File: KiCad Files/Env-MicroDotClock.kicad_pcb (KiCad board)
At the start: 2 copper layers, 90 x 65.2 mm, 48 parts, among them IC1 IS31FL3730-QFLS2-TR, IC2 IS31FL3730-QFLS2-TR, IC3 IS31FL3730-QFLS2-TR, IC4 IS31FL3730-QFLS2-TR, M1 Dip-14 Socket, M2 Dip-14 Socket, M3 Dip-14 Socket, M4 Dip-14 Socket, M5 Dip-14 Socket, M6 Dip-14 Socket, M7 Dip-14 Socket, M8 Dip-14 Socket, Q1 2SC1815, SW1 SKRK, SW2 SKRK, SW3 SKRK, SW4 SKRK, U1 Raspberry Pi Pico, U3 DS3231M

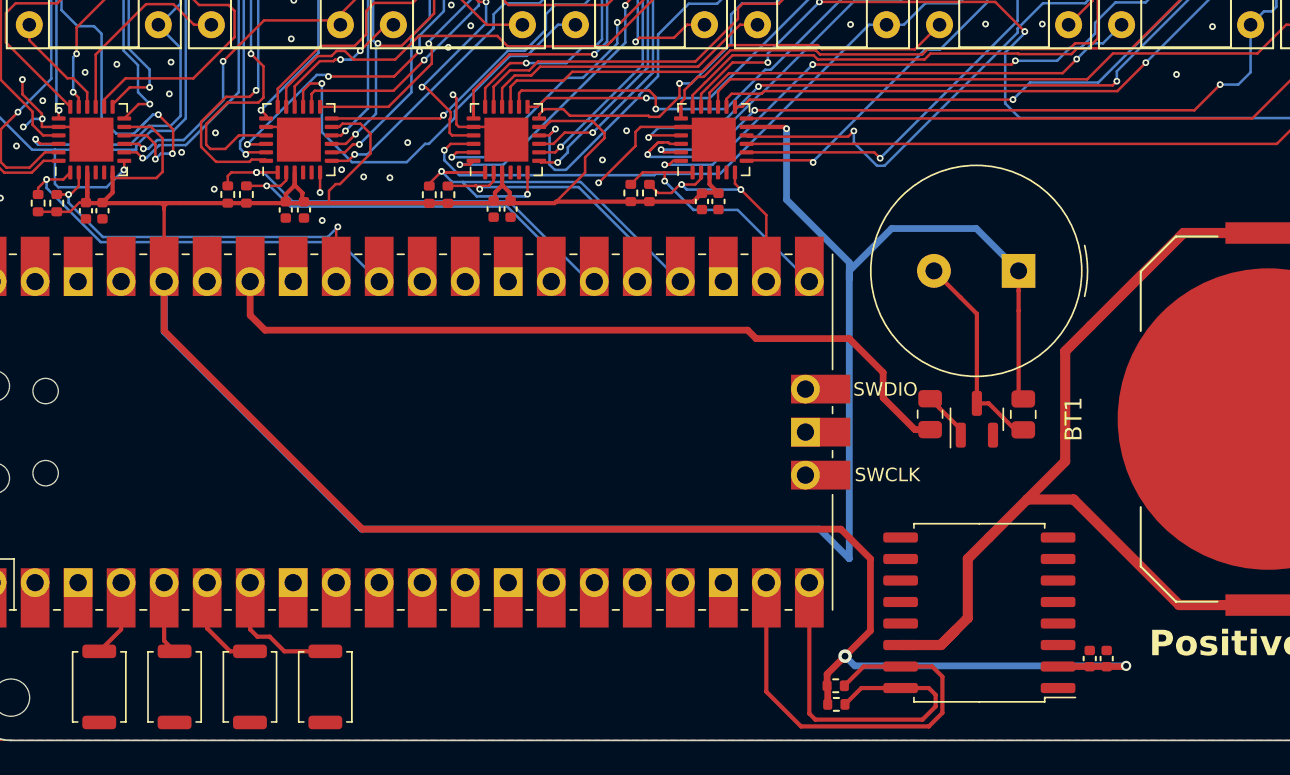
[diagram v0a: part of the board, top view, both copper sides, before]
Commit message: small tweaks + generated production files
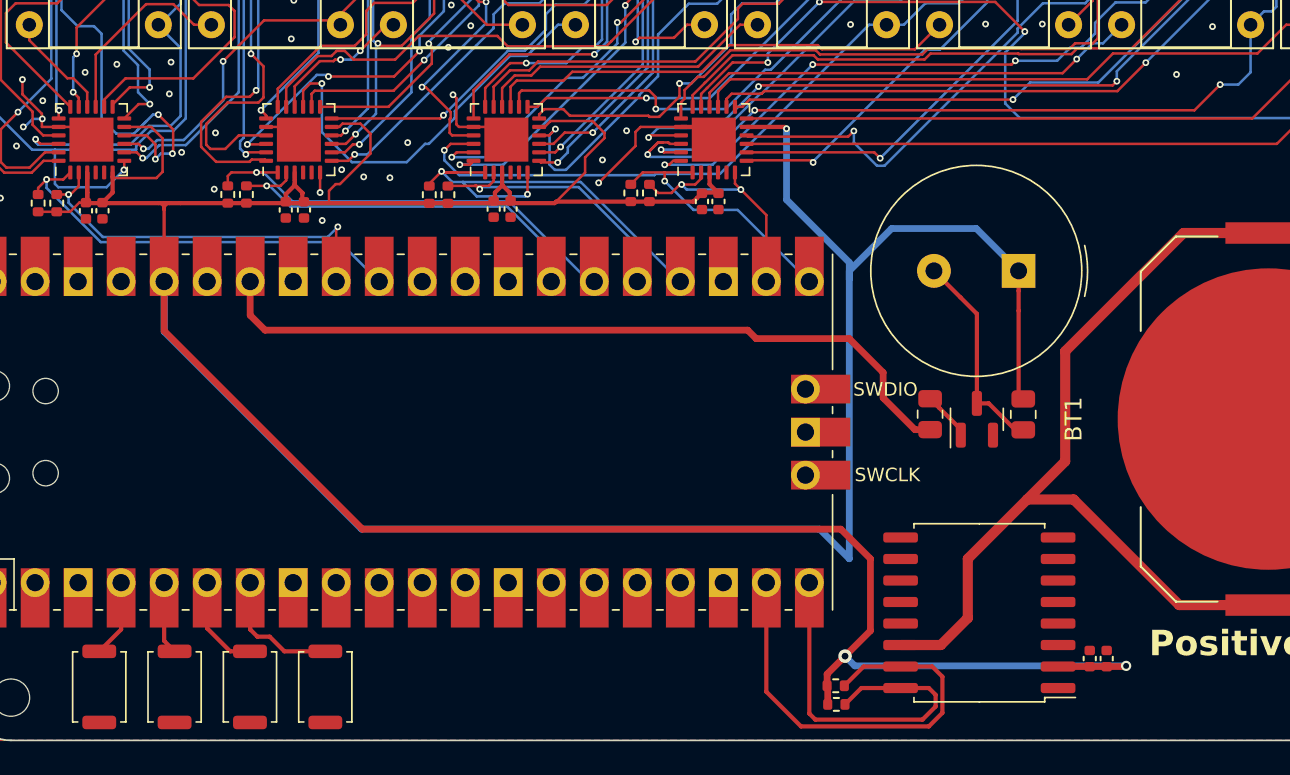
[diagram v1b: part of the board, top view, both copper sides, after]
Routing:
- net IC3C5: track 52.3 -> 50.6 mm
- net Net-(BT1-+): track 55.7 -> 54.5 mm
- net Buzzer GPIO: track 46.9 -> 45.9 mm
- net IC4C5: track 66.4 -> 65.5 mm
- net I2C2_SDA: vias 2 -> 1
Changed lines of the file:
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@@
   (segment (start 139.2 72.845) (end 136.309 72.845) (width 0.15) (layer "F.Cu") (net 46))
   (segment (start 119 85.45) (end 120.1128 85.45) (width 0.15) (layer "F.Cu") (net 46))
-  (segment (start 118.6875 85.9999) (end 118.6875 86) (width 0.15) (layer "F.Cu") (net 46))
   (segment (start 136.309 72.845) (end 134.903 74.2513) (width 0.15) (layer "F.Cu") (net 46))
   (segment (start 120.1128 85.45) (end 120.5 85.8372) (width 0.15) (layer "F.Cu") (net 46))
@@
   (segment (start 138.810736 67.765) (end 139.2 67.765) (width 0.15) (layer "F.Cu") (net 53))
   (segment (start 149.595 72.845) (end 143.25 66.5) (width 0.15) (layer "F.Cu") (net 53))
-  (segment (start 114.8125 86) (end 114.8125 85.079218) (width 0.15) (layer "F.Cu") (net 53))
   (segment (start 116.933007 82.2129) (end 114.8125 84.333407) (width 0.15) (layer "F.Cu") (net 53))
   (segment (start 114.8125 84.333407) (end 114.8125 86) (width 0.15) (layer "F.Cu") (net 53))
   (segment (start 121.9476 82.2129) (end 116.933007 82.2129) (width 0.15) (layer "F.Cu") (net 53))
   (segment (start 143.25 66.5) (end 141.5658 66.5) (width 0.15) (layer "F.Cu") (net 53))
-  (segment (start 114.812 85.3097) (end 114.8125 85.3102) (width 0.15) (layer "F.Cu") (net 53))
   (segment (start 132.450736 74.125) (end 138.810736 67.765) (width 0.15) (layer "F.Cu") (net 53))
-  (segment (start 114.8125 85.3102) (end 114.8125 86) (width 0.15) (layer "F.Cu") (net 53))
   (segment (start 121.95 82.2153) (end 121.9476 82.2129) (width 0.15) (layer "F.Cu") (net 53))
   (segment (start 141.5658 66.5) (end 140.3008 67.765) (width 0.15) (layer "F.Cu") (net 53))
@@
   (segment (start 141.3205 82.2161) (end 141.6694 81.8672) (width 0.15) (layer "F.Cu") (net 71))
   (segment (start 150.337695 81.5612) (end 151.3888 81.5612) (width 0.15) (layer "F.Cu") (net 71))
-  (segment (start 127.0625 86) (end 127.0625 85.107006) (width 0.15) (layer "F.Cu") (net 71))
   (segment (start 153.5203 76.675) (end 158.5085 71.6868) (width 0.15) (layer "F.Cu") (net 71))
   (segment (start 160.7 67.765) (end 161.865 66.6) (width 0.15) (layer "F.Cu") (net 71))
@@
   (via (at 106.8 92.4) (size 0.4) (drill 0.2) (layers "F.Cu" "B.Cu") (net 84))
   (via (at 90.9 90.49) (size 0.4) (drill 0.2) (layers "F.Cu" "B.Cu") (net 84))
-  (segment (start 99.4 93) (end 92.924264 93) (width 0.15) (layer "B.Cu") (net 84))
+  (segment (start 92.924264 93) (end 106.2 93) (width 0.15) (layer "B.Cu") (net 84))
   (segment (start 106.2 93) (end 106.8 92.4) (width 0.15) (layer "B.Cu") (net 84))
   (segment (start 90.9 90.975736) (end 90.9 90.49) (width 0.15) (layer "B.Cu") (net 84))
-  (segment (start 99.4 93) (end 106.2 93) (width 0.15) (layer "B.Cu") (net 84))
   (segment (start 92.924264 93) (end 90.9 90.975736) (width 0.15) (layer "B.Cu") (net 84))
   (segment (start 100.5125 89.1875) (end 100.3 89.4) (width 0.15) (layer "F.Cu") (net 85))
   (segment (start 100.3 89.4) (end 100.3 89.98) (width 0.15) (layer "F.Cu") (net 85))
   (segment (start 103.25 89.1875) (end 100.5125 89.1875) (width 0.15) (layer "F.Cu") (net 85))
-  (via (at 102 89.1875) (size 0.4) (drill 0.2) (layers "F.Cu" "B.Cu") (net 85))
   (via (at 102 89.1875) (size 0.4) (drill 0.2) (layers "F.Cu" "B.Cu") (net 85))
   (segment (start 102.0125 89.2) (end 102 89.1875) (width 0.15) (layer "B.Cu") (net 85))
@@
   (segment (start 91.925 91) (end 92 91) (width 0.25) (layer "F.Cu") (net 95))
   (segment (start 104.25 89.8254) (end 104.25 89.65) (width 0.25) (layer "F.Cu") (net 95))
-  (segment (start 128.22 90.5) (end 128.3 90.42) (width 0.15) (layer "F.Cu") (net 95))
   (segment (start 128.0053 90.6997) (end 128.0203 90.6997) (width 0.15) (layer "F.Cu") (net 95))
   (segment (start 116.95 90.87) (end 116.95 91) (width 0.25) (layer "F.Cu") (net 95))
@@
   (segment (start 96.5424 95.631) (end 96.5424 91.375) (width 0.2) (layer "F.Cu") (net 95))
   (segment (start 92.9 90.97) (end 93.5 90.37) (width 0.25) (layer "F.Cu") (net 95))
-  (segment (start 146.9997 94.9999) (end 146.9997 94.9998) (width 0.15) (layer "F.Cu") (net 95))
   (segment (start 119.01 86.5) (end 119.36 86.1501) (width 0.15) (layer "F.Cu") (net 95))
   (segment (start 118.688 86.5) (end 119.01 86.5) (width 0.15) (layer "F.Cu") (net 95))
@@
   (segment (start 116.5 89.925) (end 116.95 90.375) (width 0.25) (layer "F.Cu") (net 95))
   (segment (start 93.5736 89.5187) (end 96.0813 89.5187) (width 0.15) (layer "F.Cu") (net 95))
-  (segment (start 135.7275 119.4625) (end 135.69 119.5) (width 0.4) (layer "F.Cu") (net 95))
   (segment (start 103.725 91) (end 104.7 91) (width 0.25) (layer "F.Cu") (net 95))
   (segment (start 106.275 90.275) (end 106.675 89.875) (width 0.15) (layer "F.Cu") (net 95))
@@
   (segment (start 135.69 118.81) (end 135.69 119.5) (width 0.4) (layer "F.Cu") (net 95))
   (segment (start 93.5 89.4451) (end 93.5 89.1875) (width 0.25) (layer "F.Cu") (net 95))
-  (segment (start 146.9997 94.9998) (end 146.9997 94.9999) (width 0.25) (layer "F.Cu") (net 95))
   (segment (start 124.1 90.91) (end 125.2 90.91) (width 0.25) (layer "F.Cu") (net 95))
   (segment (start 127.795 90.91) (end 128.0053 90.6997) (width 0.25) (layer "F.Cu") (net 95))
@@
   (segment (start 135.25 110.25) (end 108.2 110.25) (width 0.4) (layer "B.Cu") (net 95))
   (segment (start 144 112) (end 144 115.5) (width 0.6) (layer "F.Cu") (net 101))
-  (segment (start 151.25 98.25) (end 149.75 99.75) (width 0.6) (layer "F.Cu") (net 101))
-  (segment (start 144 115.5) (end 142.406 117.094) (width 0.6) (layer "F.Cu") (net 101))
+  (segment (start 149.75 99.75) (end 156.735 92.765) (width 0.6) (layer "F.Cu") (net 101))
+  (segment (start 142.406 117.094) (end 144 115.5) (width 0.6) (layer "F.Cu") (net 101))
   (segment (start 150.25 108.5) (end 156.485 114.735) (width 0.6) (layer "F.Cu") (net 101))
-  (segment (start 145.25 110.75) (end 144 112) (width 0.6) (layer "F.Cu") (net 101))
-  (segment (start 149.75 104.75) (end 149.75 106.25) (width 0.6) (layer "F.Cu") (net 101))
-  (segment (start 156.735 92.765) (end 151.25 98.25) (width 0.6) (layer "F.Cu") (net 101))
+  (segment (start 144 112) (end 147.5 108.5) (width 0.6) (layer "F.Cu") (net 101))
+  (segment (start 149.75 99.75) (end 149.75 106.25) (width 0.6) (layer "F.Cu") (net 101))
   (segment (start 149.75 106.25) (end 147.5 108.5) (width 0.6) (layer "F.Cu") (net 101))
   (segment (start 147.5 108.5) (end 150.25 108.5) (width 0.6) (layer "F.Cu") (net 101))
-  (segment (start 149.75 99.75) (end 149.75 104.75) (width 0.6) (layer "F.Cu") (net 101))
   (segment (start 142.406 117.094) (end 140.0304 117.094) (width 0.6) (layer "F.Cu") (net 101))
-  (segment (start 142.406 117.094) (end 143.25 116.25) (width 0.6) (layer "F.Cu") (net 101))
   (segment (start 156.485 114.735) (end 161.75 114.735) (width 0.6) (layer "F.Cu") (net 101))
-  (segment (start 147.5 108.5) (end 145.25 110.75) (width 0.6) (layer "F.Cu") (net 101))
   (segment (start 161.75 92.765) (end 156.735 92.765) (width 0.6) (layer "F.Cu") (net 101))
   (segment (start 142.0457 102.8228) (end 141.7737 102.5508) (width 0.25) (layer "F.Cu") (net 103))
@@
   (segment (start 143.5867 104.6956) (end 143.5867 104.6982) (width 0.15) (layer "F.Cu") (net 103))
   (segment (start 143.5867 104.6588) (end 143.5867 104.6798) (width 0.15) (layer "F.Cu") (net 103))
-  (segment (start 101.622 95.6643) (end 101.622 95.6476) (width 0.15) (layer "F.Cu") (net 104))
   (segment (start 101.622 95.6476) (end 101.622 95.631) (width 0.15) (layer "F.Cu") (net 104))
   (segment (start 131.5 99) (end 131 98.5) (width 0.4) (layer "F.Cu") (net 104))
-  (segment (start 101.622 95.8974) (end 101.622 95.7642) (width 0.15) (layer "F.Cu") (net 104))
   (segment (start 137 99) (end 131.5 99) (width 0.4) (layer "F.Cu") (net 104))
-  (segment (start 101.622 95.7642) (end 101.622 95.6976) (width 0.15) (layer "F.Cu") (net 104))
-  (segment (start 101.622 95.6643) (end 101.622 95.6476) (width 0.25) (layer "F.Cu") (net 104))
   (segment (start 101.622 95.6476) (end 101.622 95.631) (width 0.25) (layer "F.Cu") (net 104))
-  (segment (start 101.622 96.1642) (end 101.622 96.1638) (width 0.15) (layer "F.Cu") (net 104))
   (segment (start 102.5 98.5) (end 101.6224 97.6224) (width 0.4) (layer "F.Cu") (net 104))
   (segment (start 101.6224 97.6224) (end 101.6224 95.631) (width 0.4) (layer "F.Cu") (net 104))
-  (segment (start 101.622 96.1642) (end 101.622 96.1638) (width 0.25) (layer "F.Cu") (net 104))
   (segment (start 139 102.5) (end 139 101) (width 0.4) (layer "F.Cu") (net 104))
   (segment (start 101.622 95.6476) (end 101.6224 95.6472) (width 0.15) (layer "F.Cu") (net 104))
   (segment (start 140.8753 104.3753) (end 139 102.5) (width 0.4) (layer "F.Cu") (net 104))
-  (segment (start 101.622 95.7642) (end 101.622 95.6976) (width 0.25) (layer "F.Cu") (net 104))
   (segment (start 131 98.5) (end 102.5 98.5) (width 0.4) (layer "F.Cu") (net 104))
-  (segment (start 101.622 95.6976) (end 101.622 95.6643) (width 0.15) (layer "F.Cu") (net 104))
-  (segment (start 101.622 95.8974) (end 101.622 95.7642) (width 0.25) (layer "F.Cu") (net 104))
-  (segment (start 101.622 96.1638) (end 101.622 95.8974) (width 0.15) (layer "F.Cu") (net 104))
   (segment (start 141.7737 104.3753) (end 140.8753 104.3753) (width 0.4) (layer "F.Cu") (net 104))
-  (segment (start 101.622 96.1638) (end 101.622 95.8974) (width 0.25) (layer "F.Cu") (net 104))
   (segment (start 139 101) (end 137 99) (width 0.4) (layer "F.Cu") (net 104))
-  (segment (start 101.622 95.6976) (end 101.622 95.6643) (width 0.25) (layer "F.Cu") (net 104))
   (segment (start 101.6224 95.6472) (end 101.6224 95.631) (width 0.15) (layer "F.Cu") (net 104))
   (segment (start 142.5 118.964) (end 142.5 121.1) (width 0.25) (layer "F.Cu") (net 105))
